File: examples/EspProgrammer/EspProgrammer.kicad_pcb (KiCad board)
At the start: 2 copper layers, 32.5 x 11 mm, 27 parts

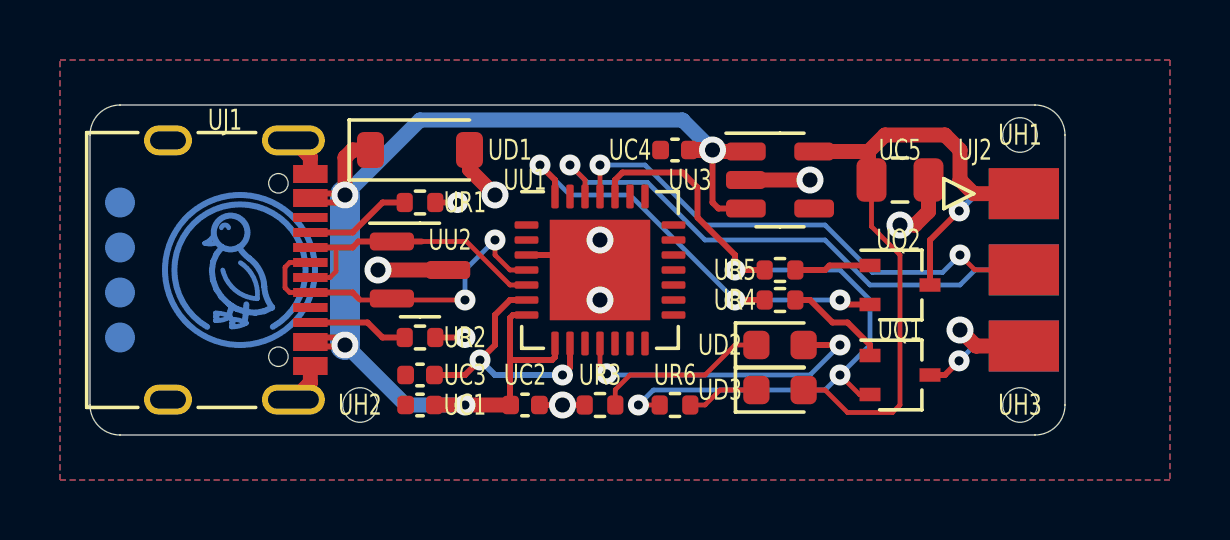
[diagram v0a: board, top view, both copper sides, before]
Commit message: cleaning
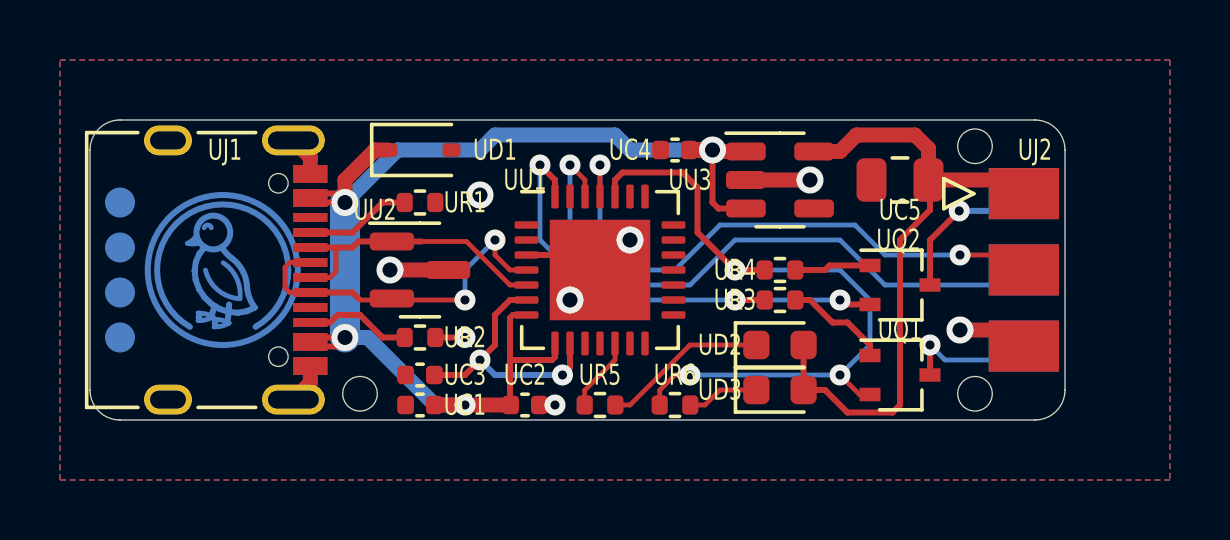
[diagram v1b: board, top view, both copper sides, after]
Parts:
- UD1: value MMSZ5232A_R1_00001 (PANJIT International) - 5?A@3V 11? Single 5.49V~5.71V 500mW 5.6V SOD-123 Zener Diodes ROHS -> BZT52-B5V6S_R1_00001 (PANJIT International) - 100nA@1V 40? Single 5.49V~5.71V 200mW 5.6V SOD-323 Zener Diodes ROHS; footprint Diode_SMD:D_SOD-123 -> Diode_SMD:D_SOD-323
- moved UH1 1.55 mm to (163.5, 43.9)
- moved UH3 1.55 mm to (163.5, 52.1)
- moved UU4 0.58 mm to (138.4, 48.0)
- moved UH2 0.38 mm to (143.0, 52.1)
- turned UC5 to 180 degrees
- renumbered UR4 to UR3, UR5 to UR4, UR3 to UR5
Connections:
- UD2 pad 2: usbconv.nsuspend -> v3v3
- UR5 pad 2: gnd -> usbconv.suspend
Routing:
- net usbconv.nsuspend: track 10.5 -> 0.00 mm, vias 2 -> 0
- net usbconv.uart.tx: track 18.3 -> 21.0 mm
- net usbconv.suspend: track 0.00 -> 2.47 mm
- net gnd: track 19.2 -> 17.4 mm, vias 10 -> 8
- net usbconv.dtr: track 15.2 -> 16.6 mm
- net usbconv.rts: track 24.8 -> 23.7 mm
- net usbconv.uart.rx: track 17.2 -> 18.2 mm
- net auto.en: track 3.53 -> 4.53 mm
- net v3v3: track 22.6 -> 21.7 mm
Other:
- board size 32.5 x 11 mm -> 32.5 x 10 mm
